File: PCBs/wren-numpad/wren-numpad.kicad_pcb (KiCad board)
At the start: 2 copper layers, 227.7 x 112.8 mm, 106 parts, among them J1 TRRS_Jack, SW0 Reset, U1 Elite-C

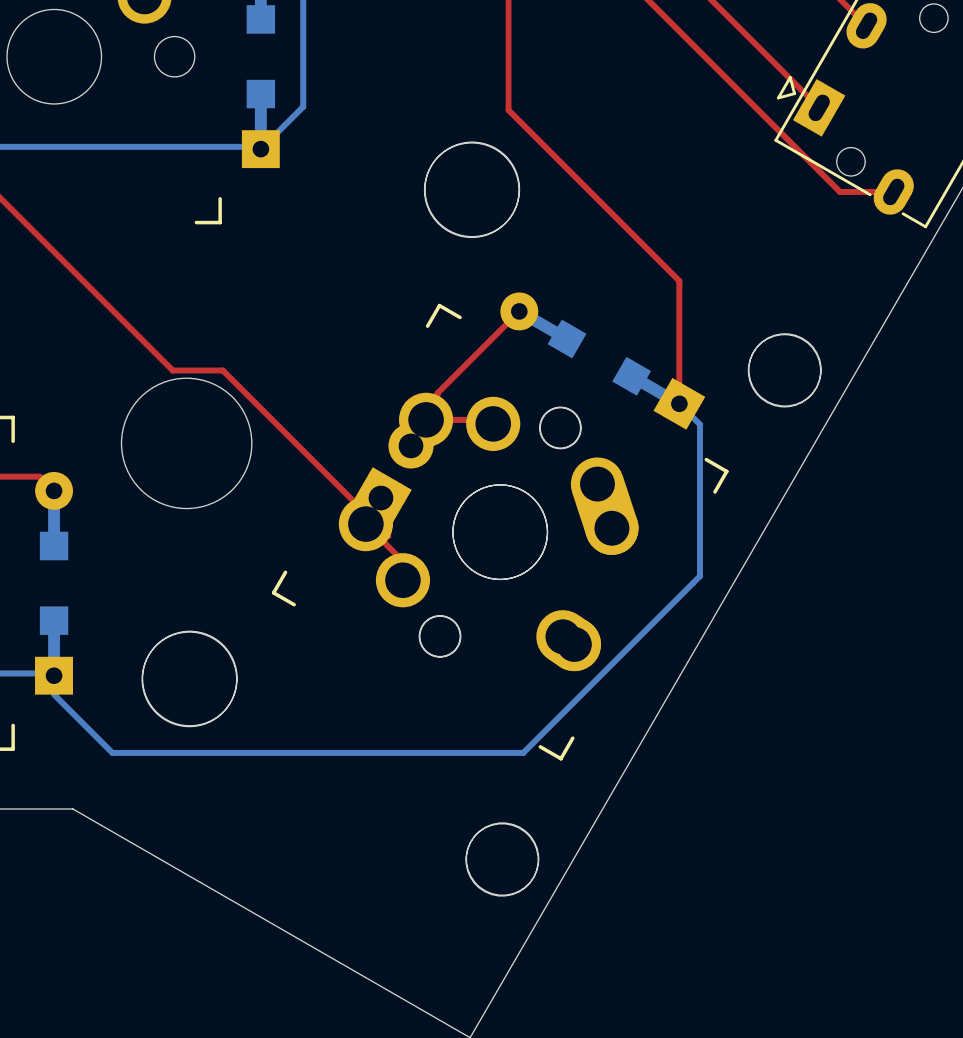
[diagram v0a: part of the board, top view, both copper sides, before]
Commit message: Wrap up remainder of system update
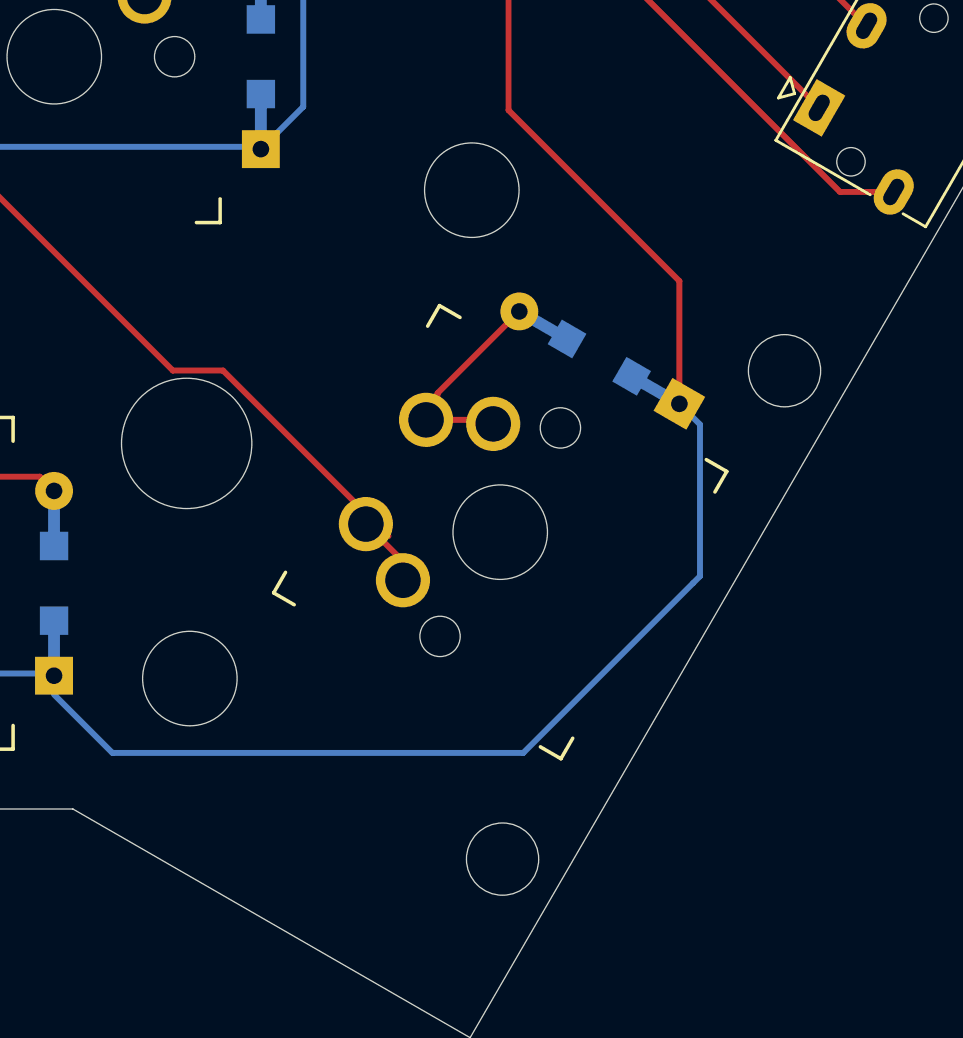
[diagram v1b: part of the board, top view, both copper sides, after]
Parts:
- removed the REF** at (239.5, 109.8)
